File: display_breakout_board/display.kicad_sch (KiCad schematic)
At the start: 8 parts, among them J1 541324562, J3 Conn_02x12_Odd_Even, U1 MCP1664T-E/OT

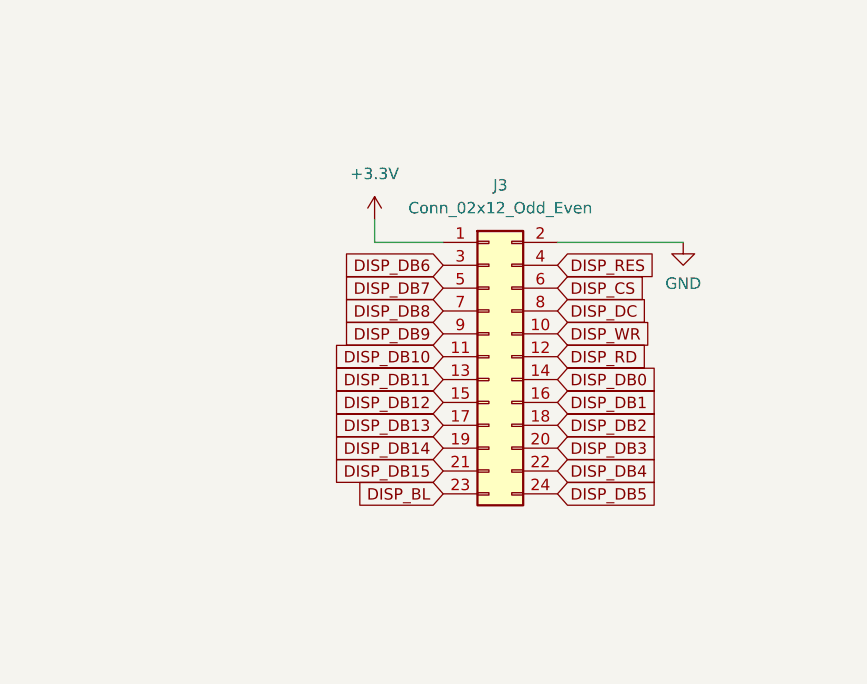
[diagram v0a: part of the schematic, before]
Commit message: Updated main PCB
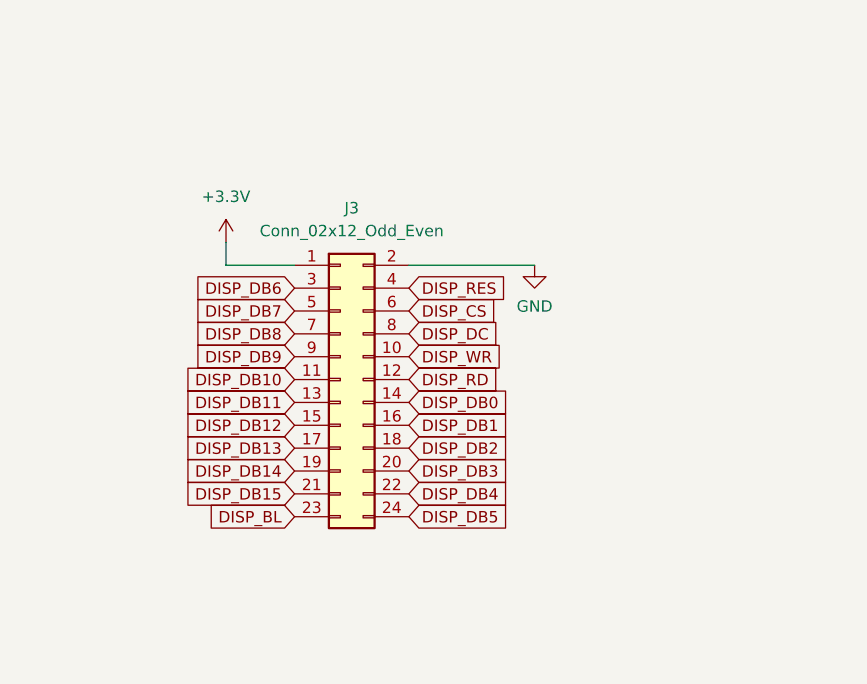
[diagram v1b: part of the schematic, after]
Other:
- moved on the sheet: J3
